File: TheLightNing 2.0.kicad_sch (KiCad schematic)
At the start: 23 parts, among them J1 motores izq, J2 motores der, J3 batt, J4 LED_izq, J5 salida a modulo, SW1 SW_SPDT, U1 L298(H)N, U2 ESP32_DEVKITC, U3 L7805

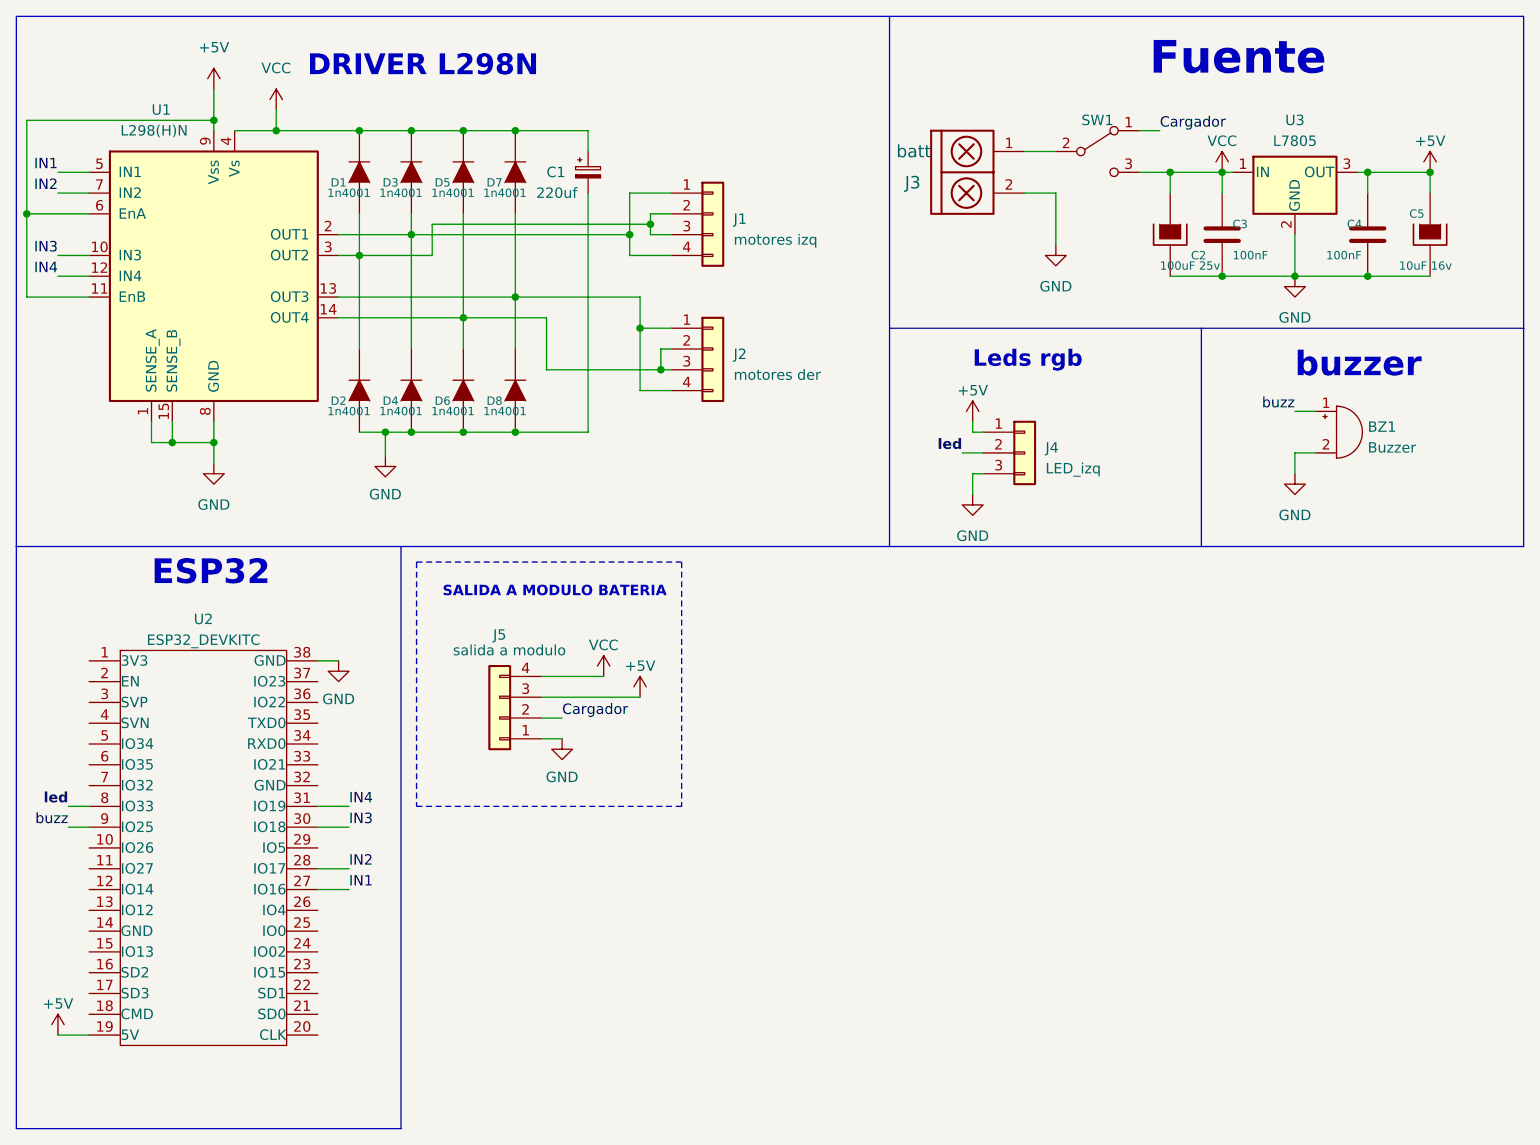
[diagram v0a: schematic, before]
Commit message: sharps
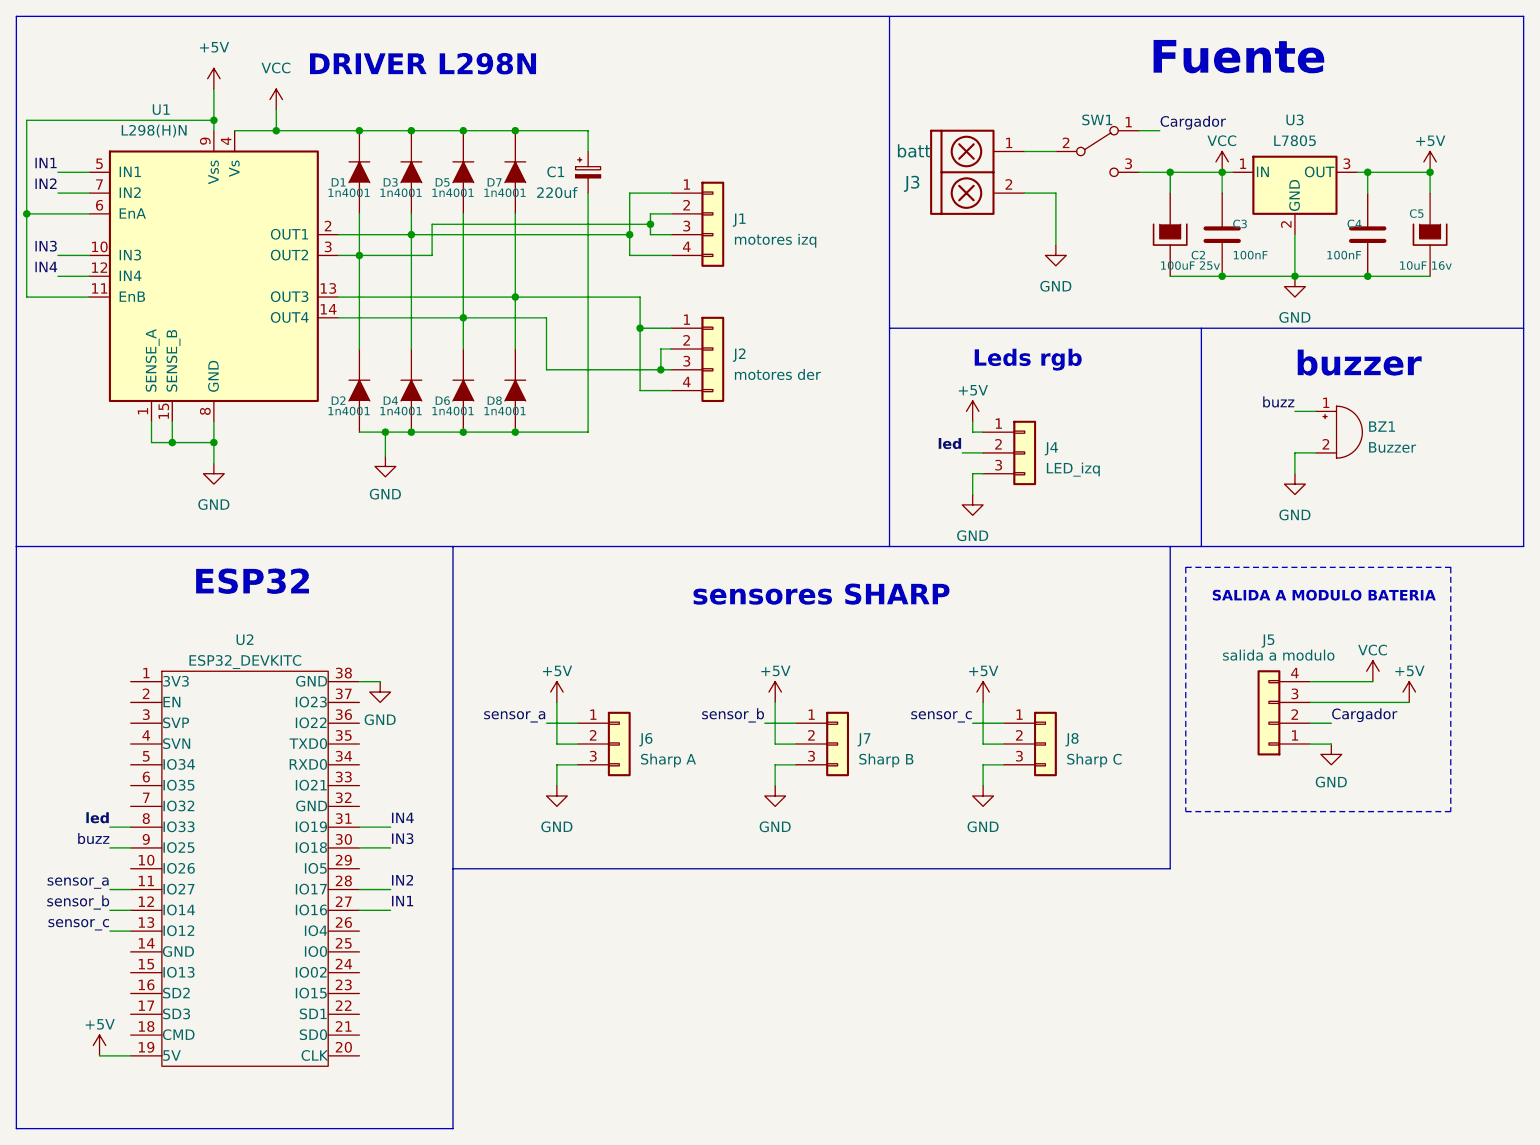
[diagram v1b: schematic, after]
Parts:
- added J6: Sharp A, EESTN5:Pin_Strip_3, symbol Connector_Generic:Conn_01x03
- added J7: Sharp B, EESTN5:Pin_Strip_3, symbol Connector_Generic:Conn_01x03
- added J8: Sharp C, EESTN5:Pin_Strip_3, symbol Connector_Generic:Conn_01x03
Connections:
- net +5V: now also J6.2 (Pin_2), J7.2 (Pin_2), J8.2 (Pin_2)
- net GND: now also J6.3 (Pin_3), J7.3 (Pin_3), J8.3 (Pin_3)
- net sensor_a: now reaches U2.11 (IO27)
- net sensor_a: now also J6.1 (Pin_1)
- net sensor_b: now reaches U2.12 (IO14)
- net sensor_b: now also J7.1 (Pin_1)
- net sensor_c: now reaches U2.13 (IO12)
- net sensor_c: now also J8.1 (Pin_1)
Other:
- note added: "sensores SHARP"
- moved on the sheet: J5, U2

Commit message: final version 1.5
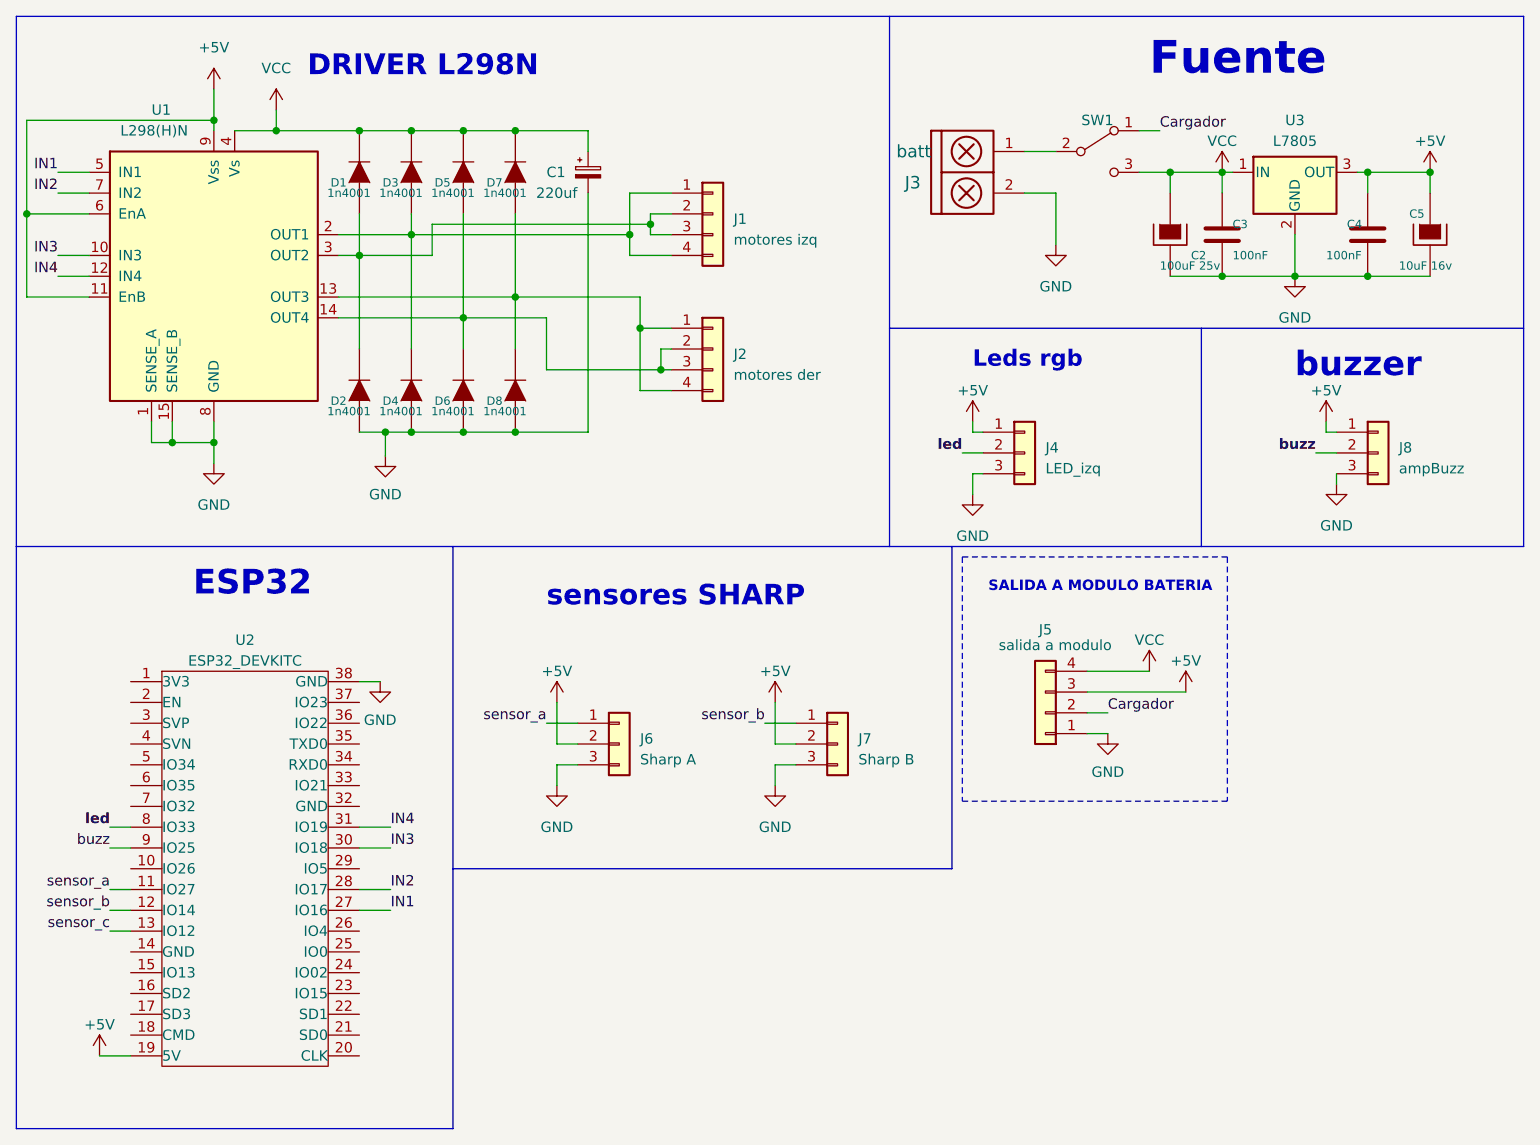
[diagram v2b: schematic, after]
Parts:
- removed BZ1: Buzzer, EESTN5:Pin_Header_2, symbol EESTN5:Buzzer
- J8: value Sharp C -> ampBuzz
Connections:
- net +5V: now also J8.1 (Pin_1); no longer J8.2 (Pin_2)
- net buzz: now also J8.2 (Pin_2)
- net sensor_c: no longer J8.1 (Pin_1)
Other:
- moved on the sheet: J5
